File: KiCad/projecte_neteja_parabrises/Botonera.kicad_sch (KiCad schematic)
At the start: 5 parts, among them SW1 SW_Push, SW2 SW_Push, SW5 SW_Rotary_1x5_MP

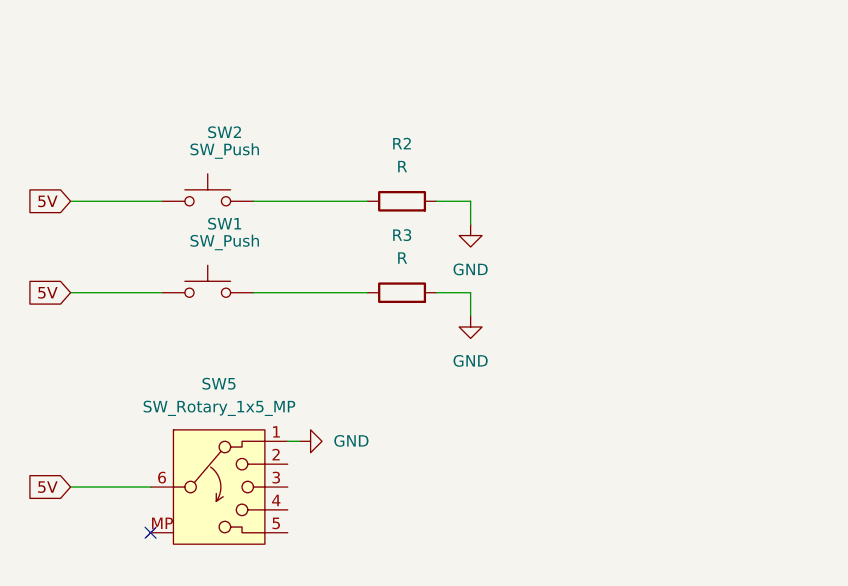
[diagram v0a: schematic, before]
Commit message: SCH V1
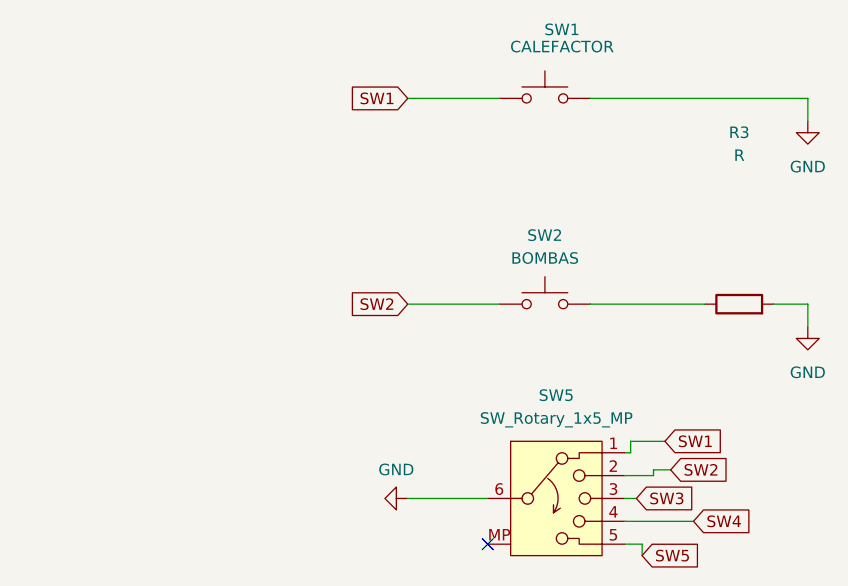
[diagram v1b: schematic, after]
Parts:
- removed R2: R, symbol Device:R
- SW1: renamed from SW2; value SW_Push -> CALEFACTOR
- SW2: renamed from SW1; value SW_Push -> BOMBAS
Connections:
- net GND: now also SW1.2, SW5.6; no longer SW5.1
- net SW2: now reaches SW5.2
- net SW2: now also SW2.1
- net SW3: now reaches SW5.3
- net SW4: now reaches SW5.4
- net SW5: now reaches SW5.5
- removed net 5V: SW1.1, SW2.1, SW5.6
- new net SW1: SW1.1, SW5.1
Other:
- moved on the sheet: R3, SW1, SW2, SW5
